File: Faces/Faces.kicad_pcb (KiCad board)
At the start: 6 copper layers, 120.8 x 142.1 mm, 156 parts

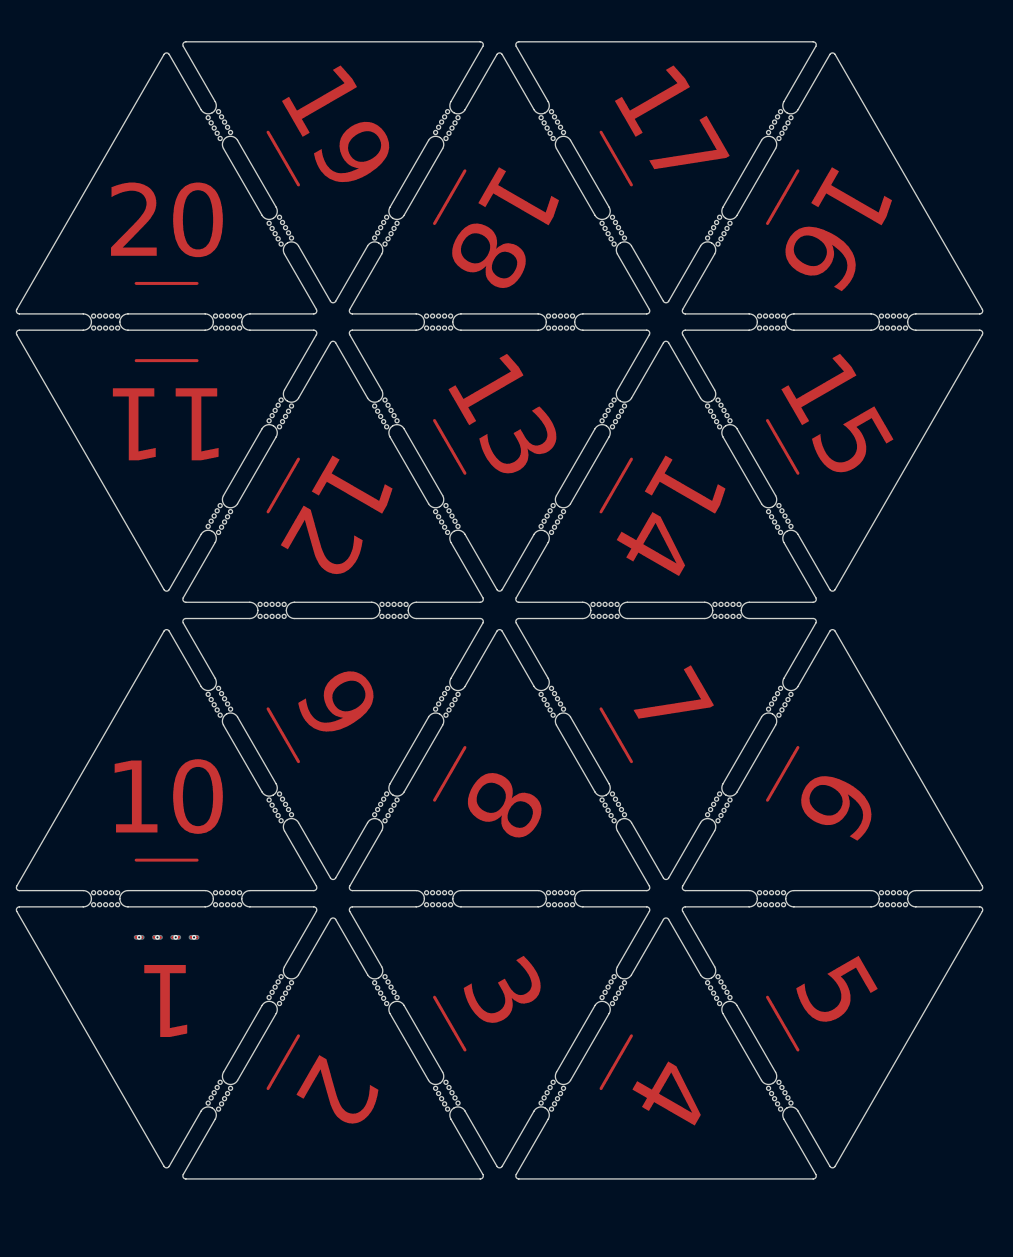
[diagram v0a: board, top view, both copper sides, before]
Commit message: Somewhere around the first complete prototype. time to change BMS
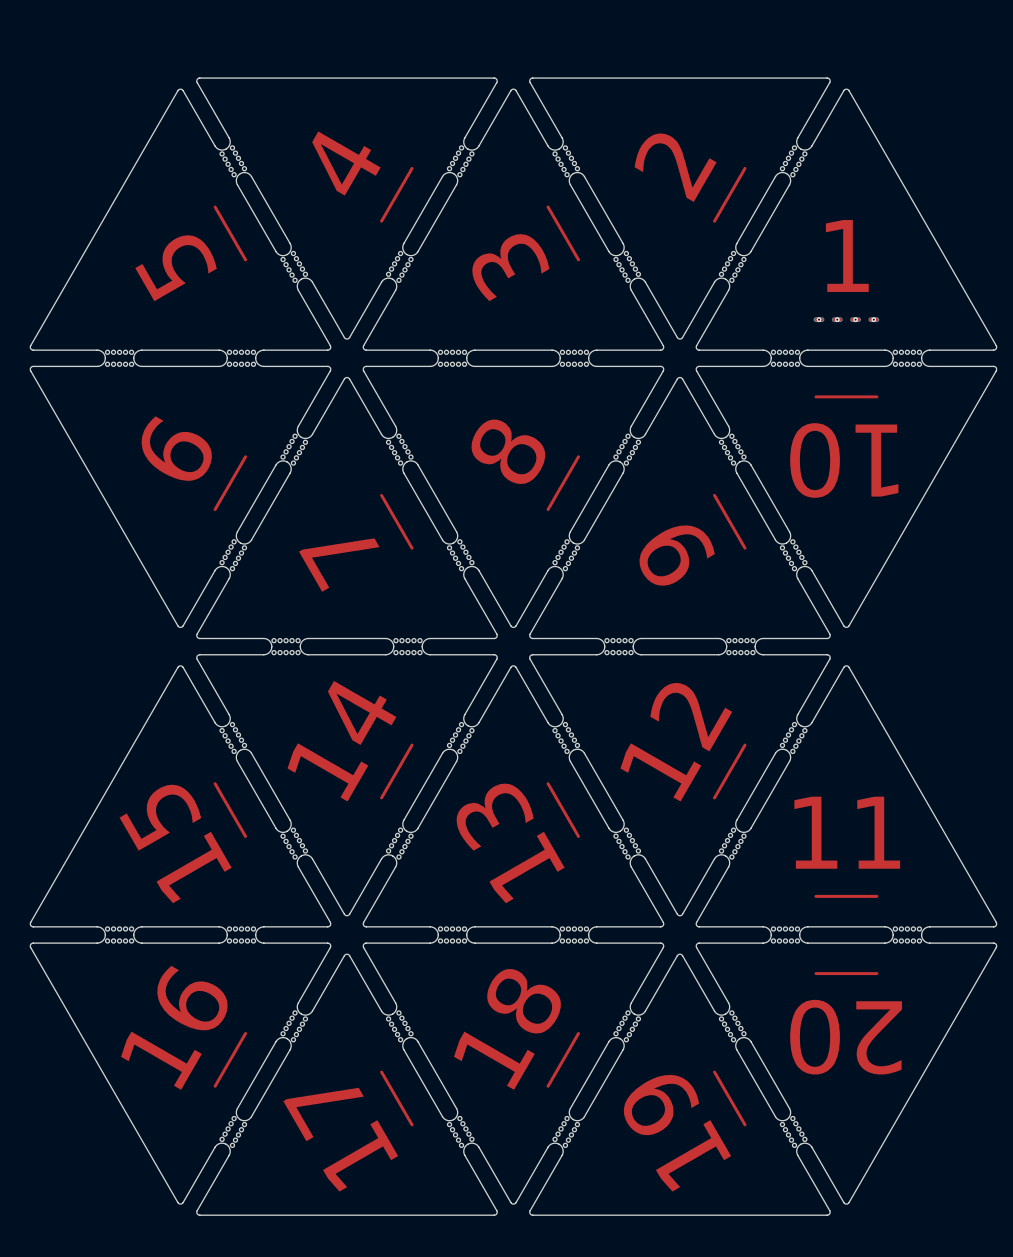
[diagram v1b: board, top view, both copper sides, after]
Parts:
- moved G*** 152.7 mm to (119.2, 161.9), turned to 115 degrees
- moved G*** 149.4 mm to (47.1, 148.8), turned to 55 degrees
- moved G*** 148.4 mm to (147.6, 140.7), turned to 170 degrees
- moved G*** 146.0 mm to (77.8, 161.5), turned to 115 degrees
- moved mouse-bite-2mm-slot 144.9 mm to (129.2, 153.1), turned to 120 degrees
- moved mouse-bite-2mm-slot 144.9 mm to (129.2, 153.1), turned to -60 degrees
- moved mouse-bite-2mm-slot 143.2 mm to (59.1, 153.1), turned to 60 degrees
- moved mouse-bite-2mm-slot 143.2 mm to (59.1, 153.1), turned to -120 degrees
- moved G*** 143.2 mm to (117.2, 22.7), turned to 115 degrees
- moved G*** 141.0 mm to (145.6, 42.8), turned to 55 degrees
- moved G*** 140.4 mm to (46.1, 38.1), turned to 175 degrees
- moved G*** 137.6 mm to (75.6, 23.7), turned to 115 degrees
- moved mouse-bite-2mm-slot 137.1 mm to (129.2, 31.7), turned to -120 degrees
- moved mouse-bite-2mm-slot 137.1 mm to (129.2, 31.7), turned to 60 degrees
- moved mouse-bite-2mm-slot 135.3 mm to (59.1, 31.7), turned to -60 degrees
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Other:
- board text added: "DIO"
- board text added: "GND"
- board text added: "SCK"
- board text added: "VBUS"
